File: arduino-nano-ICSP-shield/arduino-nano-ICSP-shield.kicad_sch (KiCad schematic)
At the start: 11 parts, among them J1 Analog, J2 Digital, J3 AVR-ISP-6, J4 Conn_02x04_Counter_Clockwise

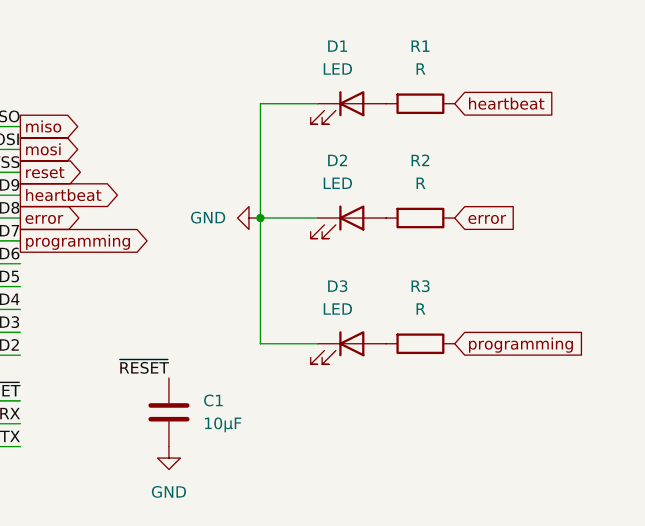
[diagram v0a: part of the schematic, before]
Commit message: continue
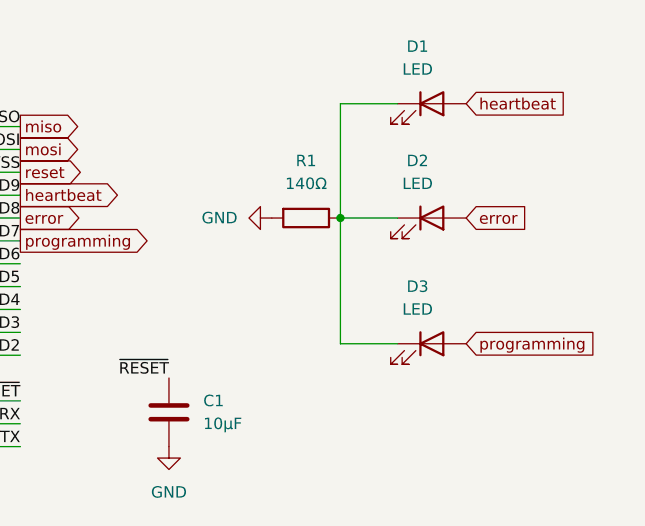
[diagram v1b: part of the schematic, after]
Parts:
- removed R2, R3: R, Resistor_SMD:R_0805_2012Metric_Pad1.20x1.40mm_HandSolder, symbol Device:R
- C1: footprint Capacitor_SMD:C_0805_2012Metric_Pad1.18x1.45mm_HandSolder -> Capacitor_SMD:C_0603_1608Metric
- D1, D2, D3: footprint LED_SMD:LED_0805_2012Metric_Pad1.15x1.40mm_HandSolder -> LED_SMD:LED_0603_1608Metric
- R1: value R -> 140Ω; footprint Resistor_SMD:R_0805_2012Metric_Pad1.20x1.40mm_HandSolder -> Resistor_SMD:R_0603_1608Metric
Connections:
- net GND: now also R1.2; no longer D1.1 (K), D2.1 (K), D3.1 (K)
- net error: now also D2.2 (A)
- net heartbeat: now also D1.2 (A); no longer R1.1
- net programming: now also D3.2 (A)
- new net: D1.1 (K), D2.1 (K), D3.1 (K), R1.1
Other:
- moved on the sheet: D1, D2, D3, R1
